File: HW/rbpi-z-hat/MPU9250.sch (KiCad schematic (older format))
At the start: 9 parts

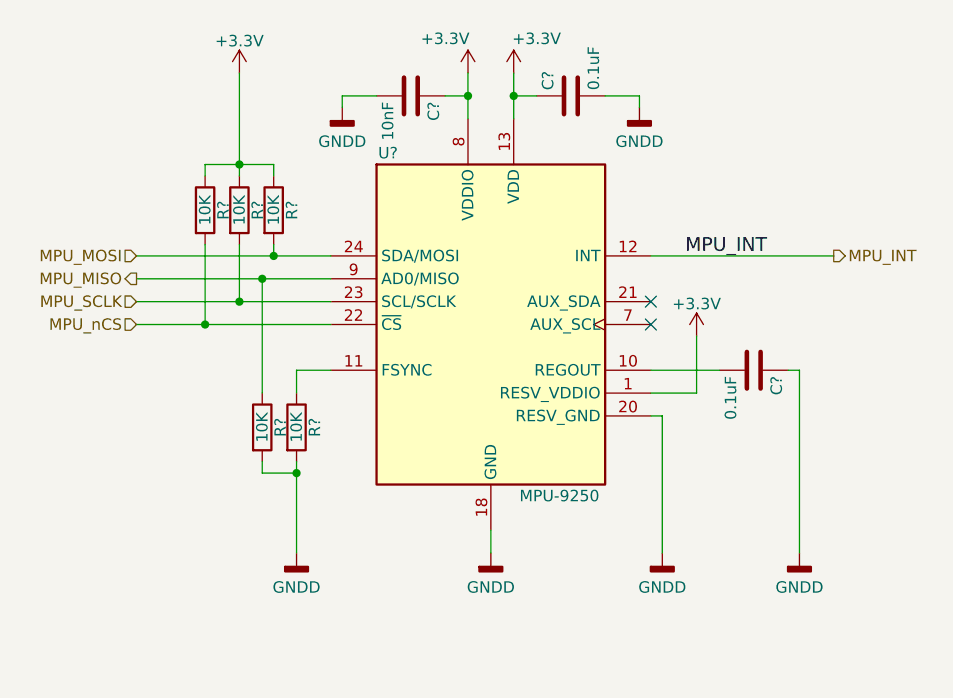
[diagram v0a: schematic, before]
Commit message: Commit...
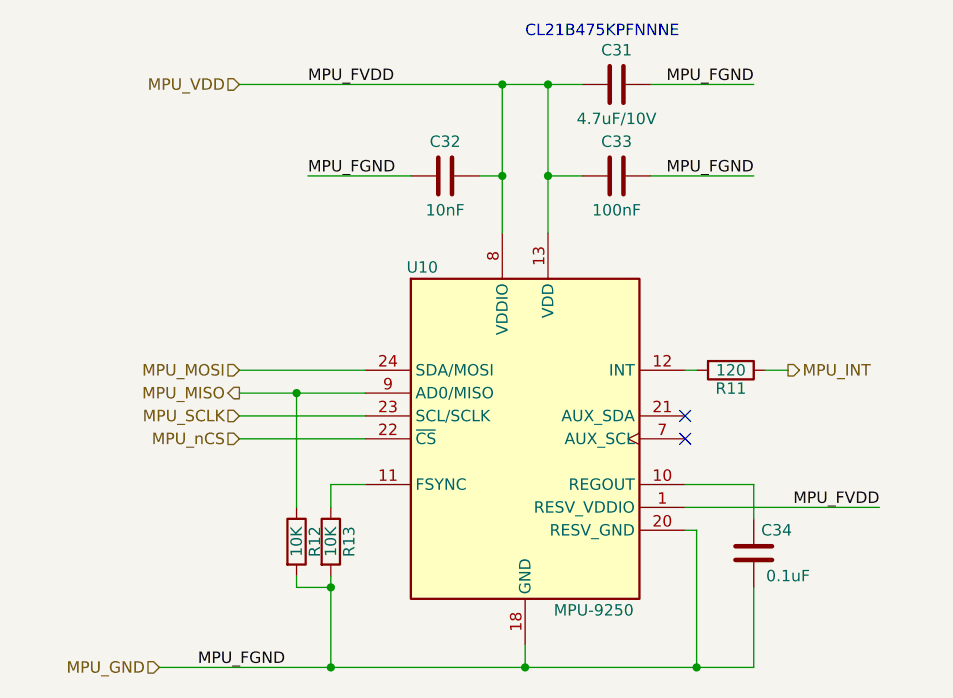
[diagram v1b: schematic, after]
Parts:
- removed C? (x2): 0.1uF, Capacitor_SMD:C_0603_1608Metric, symbol Device:C
- removed C?: 10nF, Capacitor_SMD:C_0603_1608Metric, symbol Device:C
- removed R? (x5): 10K, Resistor_SMD:R_0603_1608Metric, symbol Device:R
- removed U?: MPU-9250, Package_DFN_QFN:QFN-24-1EP_3x3mm_P0.4mm_EP1.75x1.6mm_ThermalVias, symbol Sensor_Motion:MPU-9250
- added C3: 10nF, Capacitor_SMD:C_0603_1608Metric, symbol Device:C
- added C5: 100nF, Capacitor_SMD:C_0603_1608Metric, symbol Device:C
- added C6: 4.7uF/10V, Capacitor_SMD:C_0805_2012Metric, symbol Device:C
- added C7: 0.1uF, Capacitor_SMD:C_0603_1608Metric, symbol Device:C
- added R1: 120, Resistor_SMD:R_0603_1608Metric, symbol Device:R
- added R2, R3: 10K, Resistor_SMD:R_0603_1608Metric, symbol Device:R
- added U1: MPU-9250, Package_DFN_QFN:QFN-24-1EP_3x3mm_P0.4mm_EP1.75x1.6mm, symbol Sensor_Motion:MPU-9250
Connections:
- net MPU_INT: now also R1.1
- net MPU_MISO: now also R2.1, U1.9 (AD0/MISO)
- net MPU_MOSI: now also U1.24 (SDA/MOSI)
- net MPU_SCLK: now also U1.23 (SCL/SCLK)
- net MPU_nCS: now also U1.22 (~CS)
- new net: R1.2, U1.12 (INT)
- new net: C7.2, U1.10 (REGOUT)
- new net: R3.1, U1.11 (FSYNC)
- new net MPU_GND: C3.2, C5.2, C6.2, C7.1, R2.2, R3.2, U1.18 (GND), U1.20 (RESV_GND)
- new net MPU_VDD: C3.1, C5.1, C6.1, U1.1 (RESV_VDDIO), U1.13 (VDD), U1.8 (VDDIO)
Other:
- note added: "CL21B475KPFNNNE"
